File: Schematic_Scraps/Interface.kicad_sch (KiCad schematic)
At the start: 9 parts, among them J1 Conn_01x09, J2 Cassette, U1 АОТ101АС (ILD74), U2 К555ТЛ2 (74LS14), U3 КР580ВВ51А (8251)

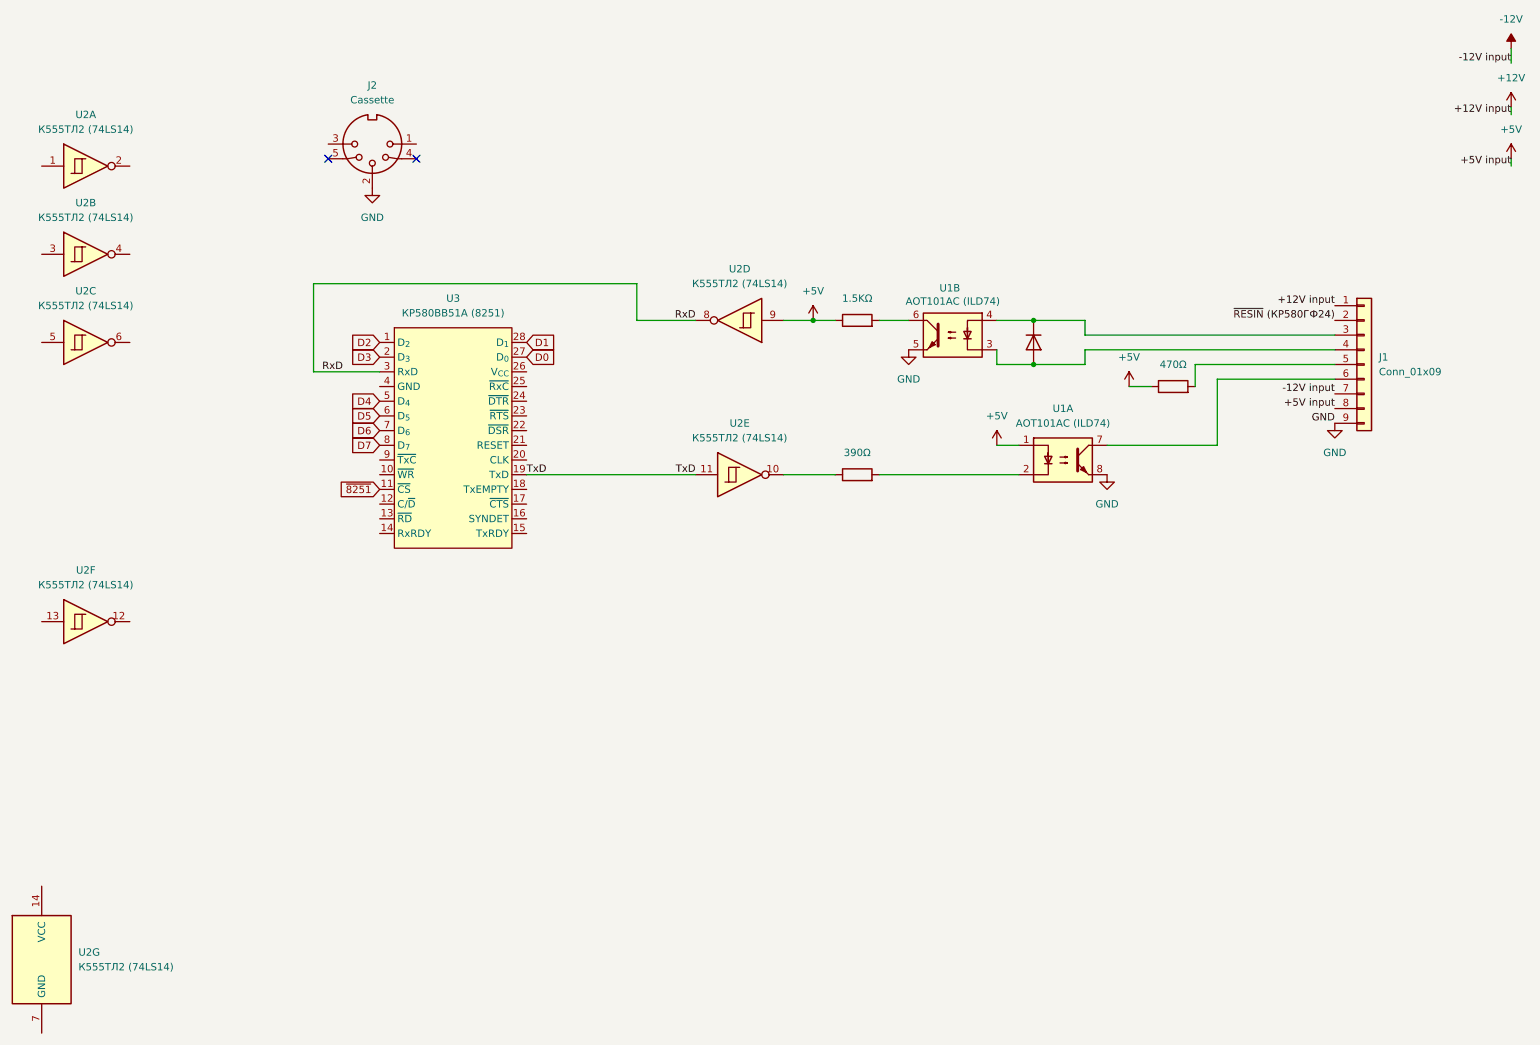
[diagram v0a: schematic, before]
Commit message: Reverse engineering progress
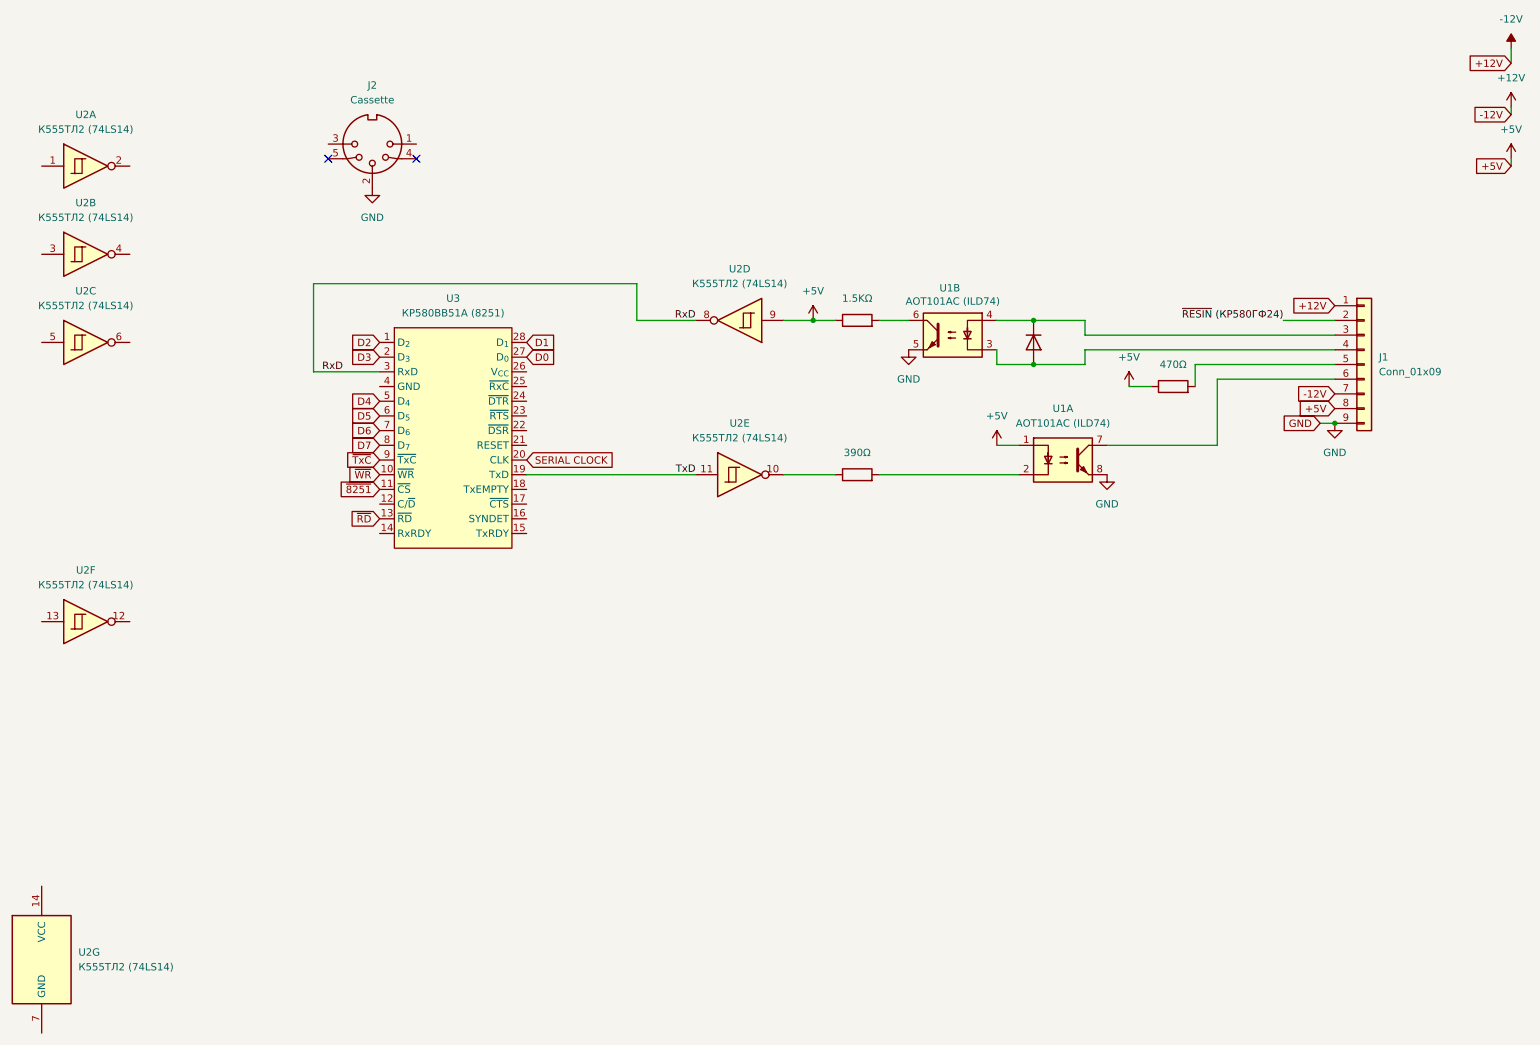
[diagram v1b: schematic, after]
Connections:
- net -12V is gone; now on net +12V: J1.7 (Pin_7)
- net ~{WR}: now reaches U3.10 (~{WR})
- net ~{RD}: now reaches U3.13 (~{RD})
- net SERIAL CLOCK: now reaches U3.20 (CLK)
- net ~{TxC}: now reaches U3.9 (~{TxC})

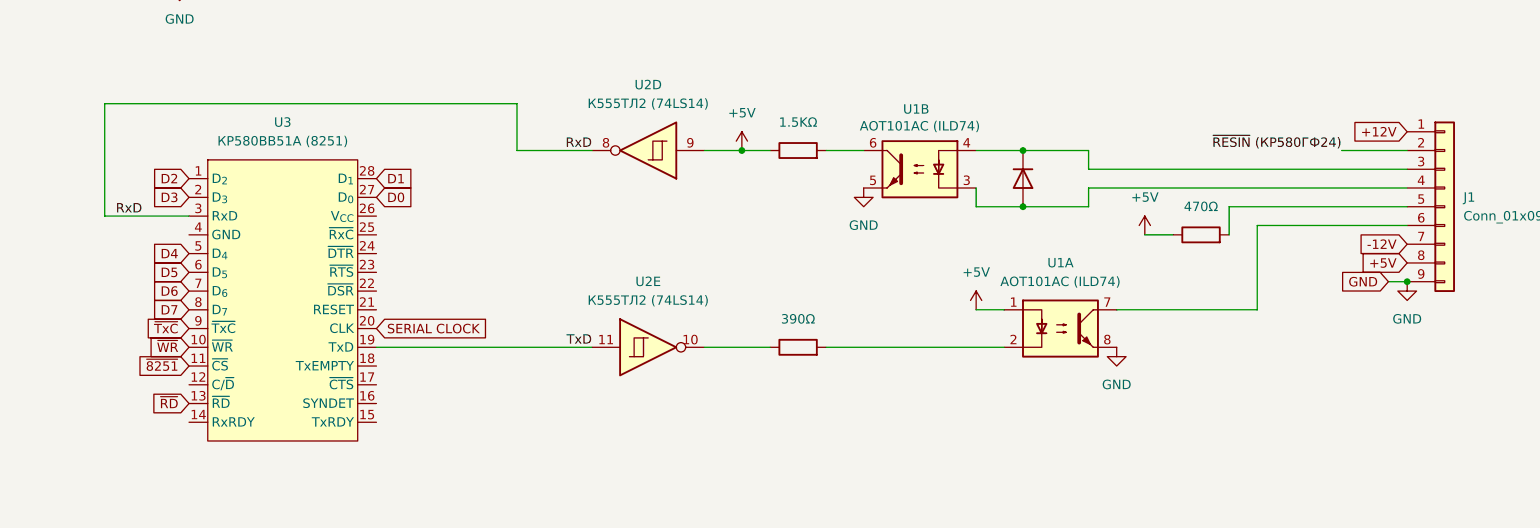
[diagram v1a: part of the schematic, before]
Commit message: Further reverse engineering progress
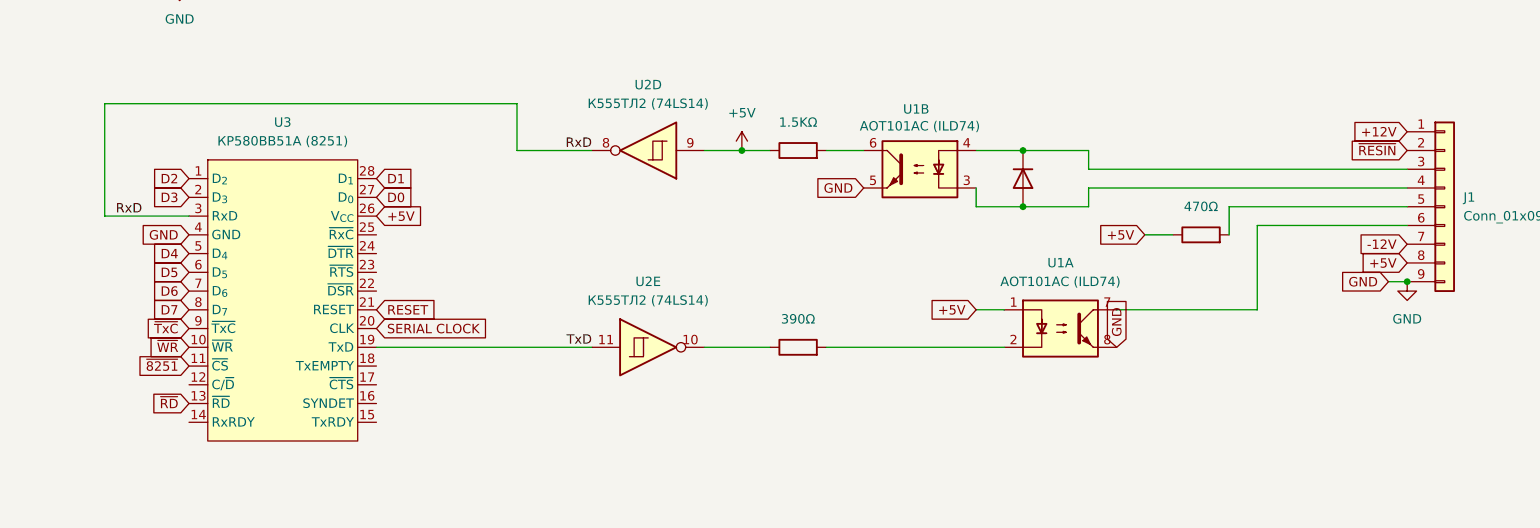
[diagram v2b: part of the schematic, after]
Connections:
- net +5V: now also U3.26 (V_{CC})
- net GND: now also U3.4 (GND)
- net RESET: now reaches U3.21 (RESET)
- net ~{RESIN} (КР580ГФ24) renamed ~{RESIN}
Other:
- company: (none) -> Brett Hallen
- title: (none) -> Rhythm Keyboard (Ритм Клав)

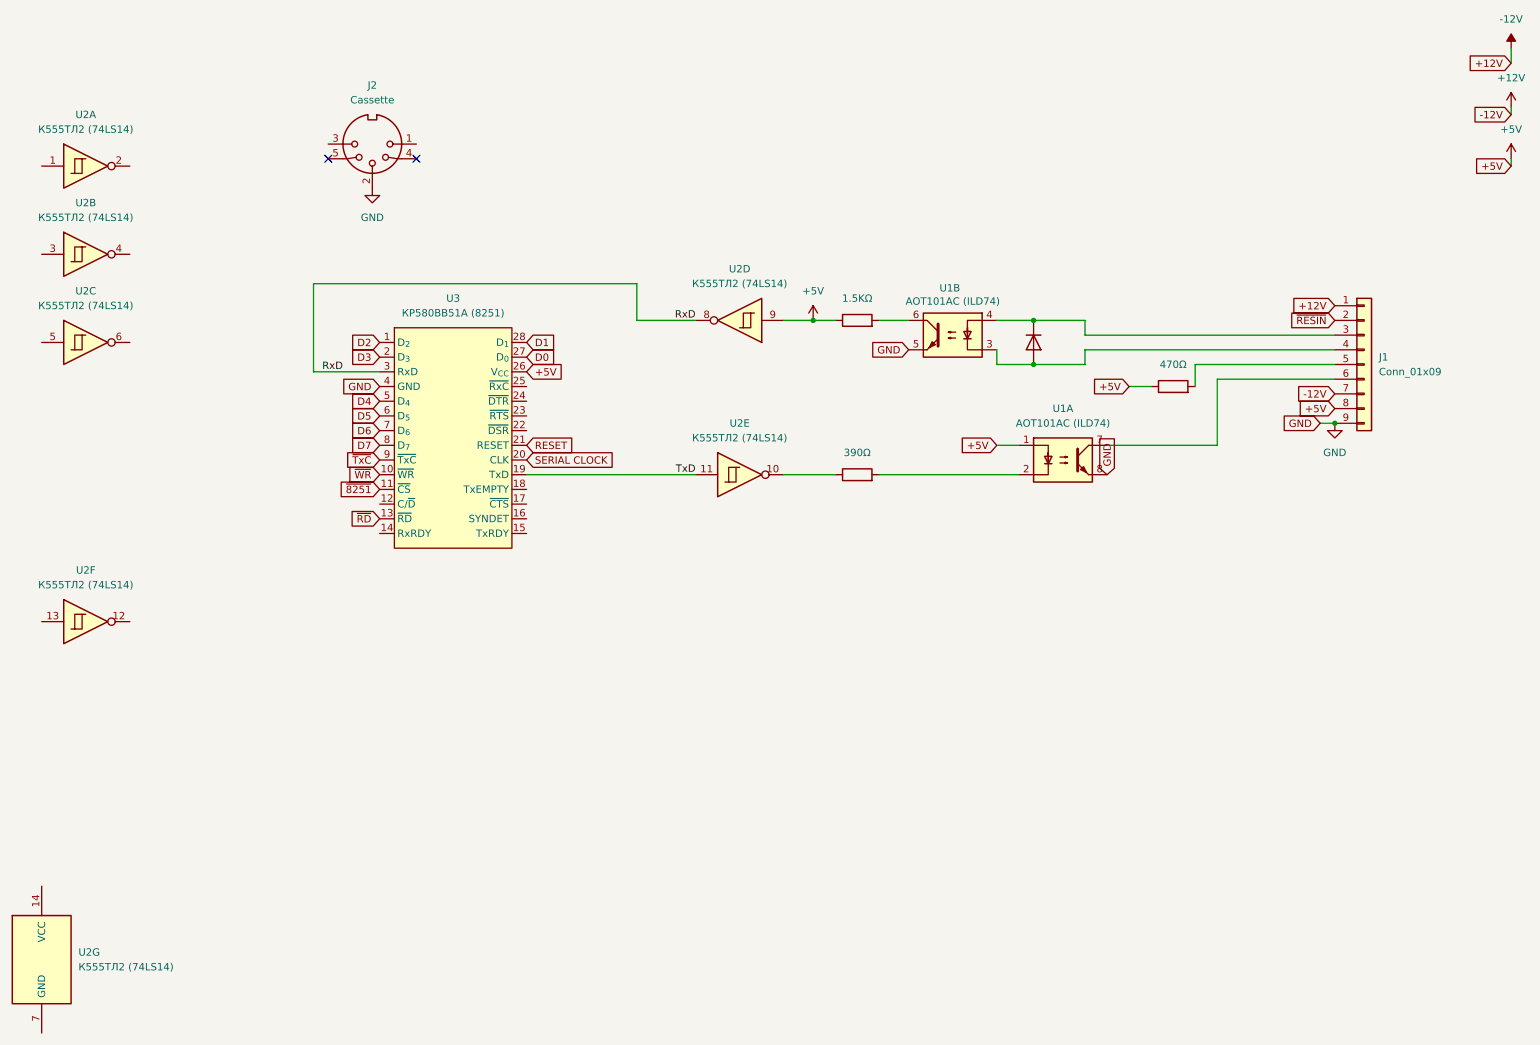
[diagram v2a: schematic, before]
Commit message: Reverse engineering updates
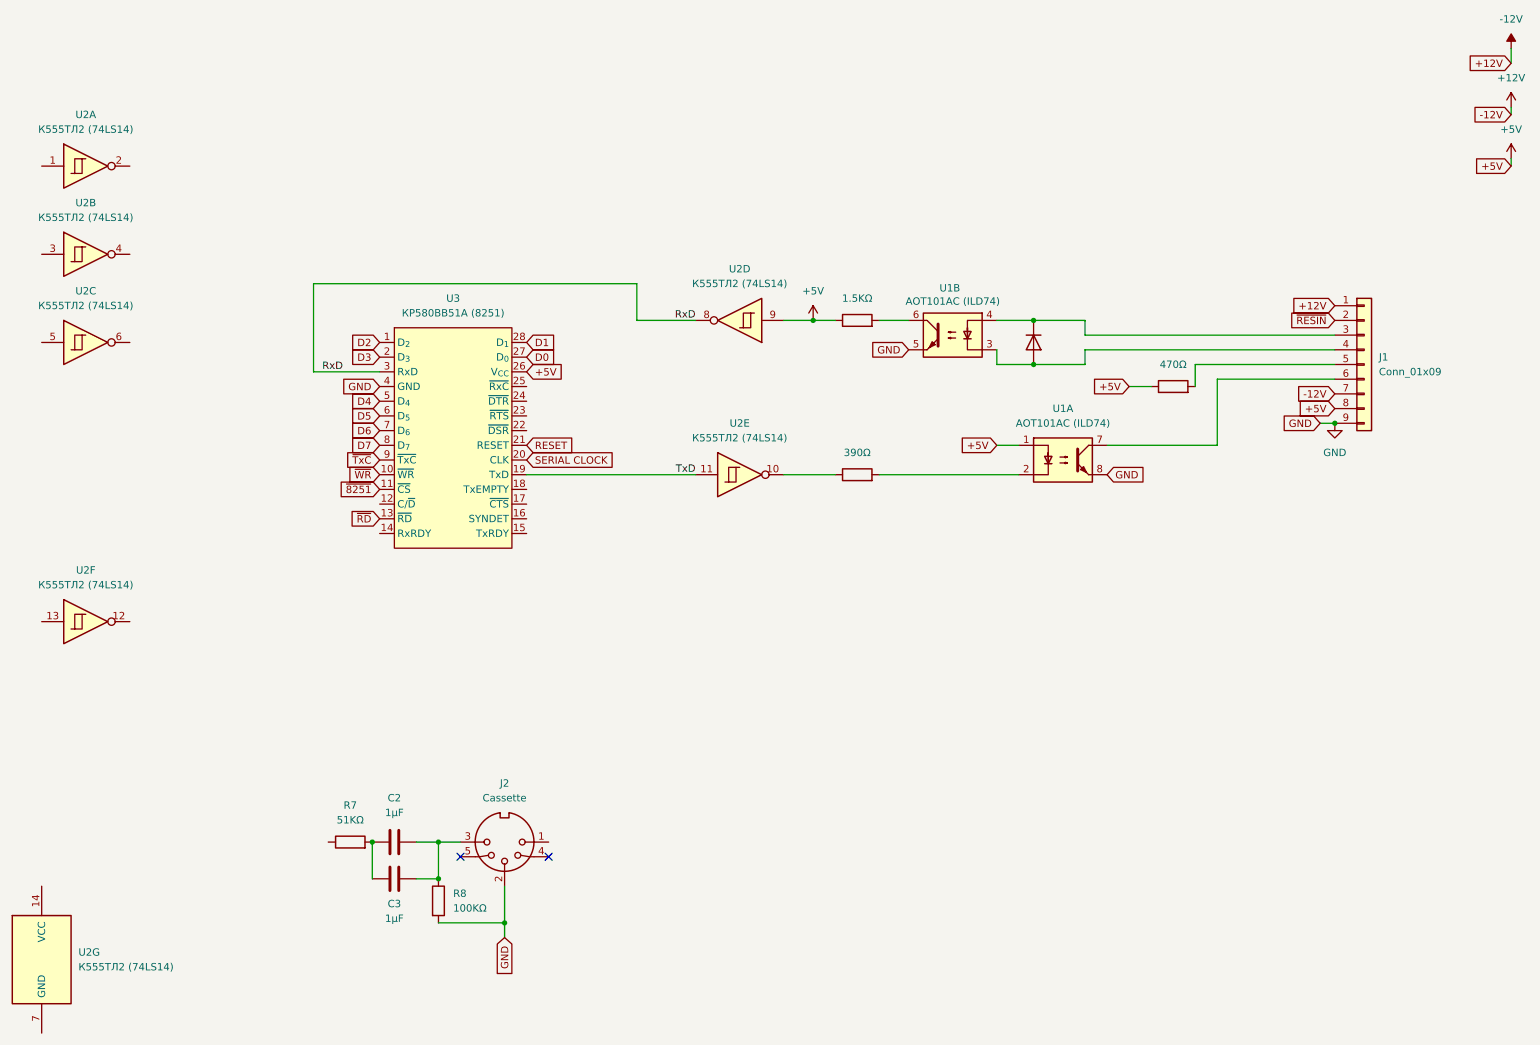
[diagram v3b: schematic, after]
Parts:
- added C2, C3: 1µF, symbol Device:C
- added R7: 51KΩ, symbol Device:R
- added R8: 100KΩ, symbol Device:R
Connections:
- net GND: now also R8.2
- net at J2.3: now also C2.2, C3.2, R8.1
- new net: C2.1, C3.1, R7.2
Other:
- moved on the sheet: J2

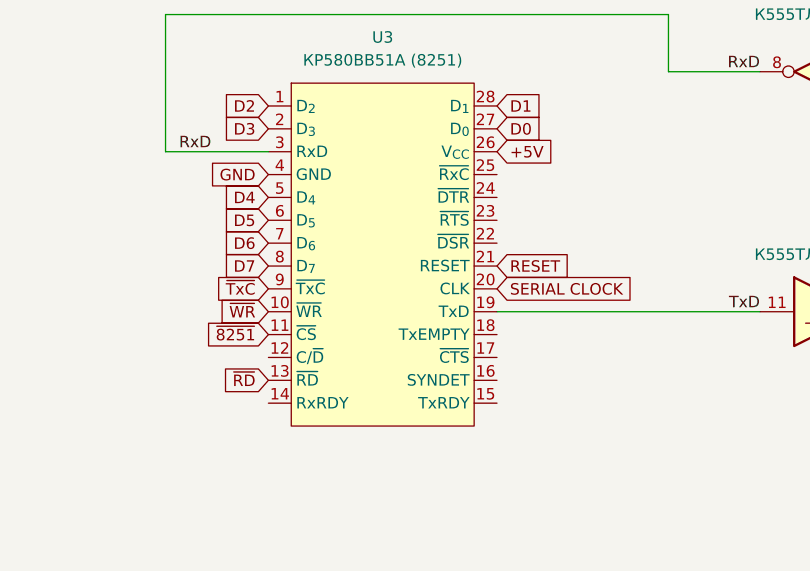
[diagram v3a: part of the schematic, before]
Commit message: 19-May reverse engineering progress
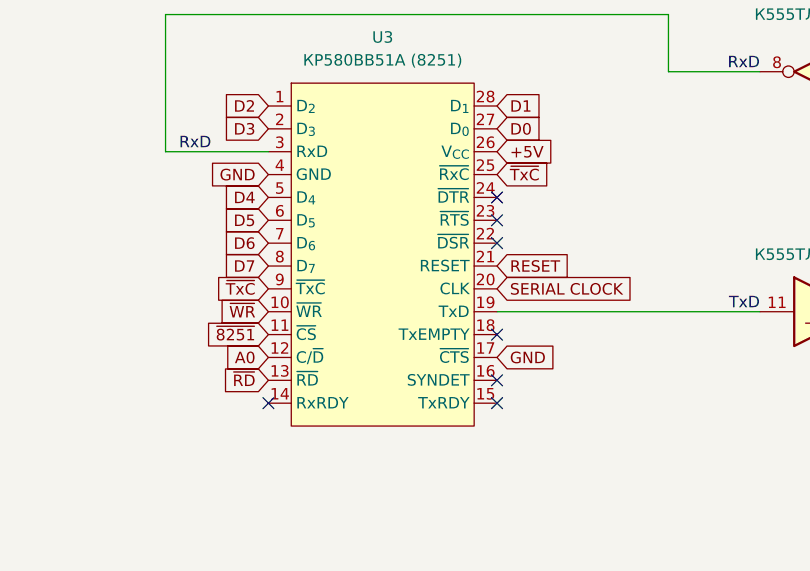
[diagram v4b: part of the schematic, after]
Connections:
- net GND: now also U3.17 (~{CTS})
- net ~{TxC}: now also U3.25 (~{RxC})
- net A0: now reaches U3.12 (C/~{D})
- no-connect marks 2 -> 9
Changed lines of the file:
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@@
 	(generator "eeschema")
 	(generator_version "9.0")
-	(paper "A4")
+	(paper "A3")
 	(title_block
 		(title "Rhythm Keyboard (Ритм Клав)")
@@
 	)
 	(no_connect
+		(at 107.95 104.14)
+	)
+	(no_connect
+		(at 107.95 83.82)
+	)
+	(no_connect
+		(at 107.95 81.28)
+	)
+	(no_connect
+		(at 107.95 101.6)
+	)
+	(no_connect
+		(at 107.95 86.36)
+	)
+	(no_connect
+		(at 82.55 104.14)
+	)
+	(no_connect
 		(at 111.76 160.02)
 	)
@@
 		(at 96.52 160.02)
 	)
+	(no_connect
+		(at 107.95 96.52)
+	)
 	(wire
 		(pts
@@
 		)
 	)
+	(global_label "A0"
+		(shape input)
+		(at 82.55 99.06 180)
+		(fields_autoplaced yes)
+		(effects
+			(font
+				(size 1.27 1.27)
+			)
+			(justify right)
+		)
+		(property "Intersheetrefs" "${INTERSHEET_REFS}"
+			(at 77.2667 99.06 0)
+			(effects
+				(font
+					(size 1.27 1.27)
+				)
+				(justify right)
+				(hide yes)
+			)
+		)
+	)
 	(global_label "D3"
 		(shape input)
@@
 		)
 	)
+	(global_label "~{TxC}"
+		(shape input)
+		(at 107.95 78.74 0)
+		(fields_autoplaced yes)
+		(effects
+			(font
+				(size 1.27 1.27)
+			)
+			(justify left)
+		)
+		(property "Intersheetrefs" "${INTERSHEET_REFS}"
+			(at 114.2009 78.74 0)
+			(effects
+				(font
+					(size 1.27 1.27)
+				)
+				(justify left)
+				(hide yes)
+			)
+		)
+	)
 	(global_label "+12V"
 		(shape input)
@@
 				(hide yes)
 			)
+		)
+	)
+	(global_label "GND"
+		(shape input)
+		(at 107.95 99.06 0)
+		(fields_autoplaced yes)
+		(effects
+			(font
+				(size 1.27 1.27)
+			)
+			(justify left)
+		)
+		(property "Intersheetrefs" "${INTERSHEET_REFS}"
+			(at 114.8057 99.06 0)
+			(effects
+				(font
+					(size 1.27 1.27)
+				)
+				(justify left)
+				(hide yes)
+			)
